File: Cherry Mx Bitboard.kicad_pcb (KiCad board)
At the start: 2 copper layers, 17.8 x 17.8 mm, 12 parts, among them P11 CONN_01X01, P12 CONN_01X01, P13 CONN_01X01, P14 CONN_01X01, P15 CONN_01X01, P16 CONN_01X01, P21 CONN_01X01, P22 CONN_01X01, P23 CONN_01X01, P24 CONN_01X01, SW1 SW_PUSH

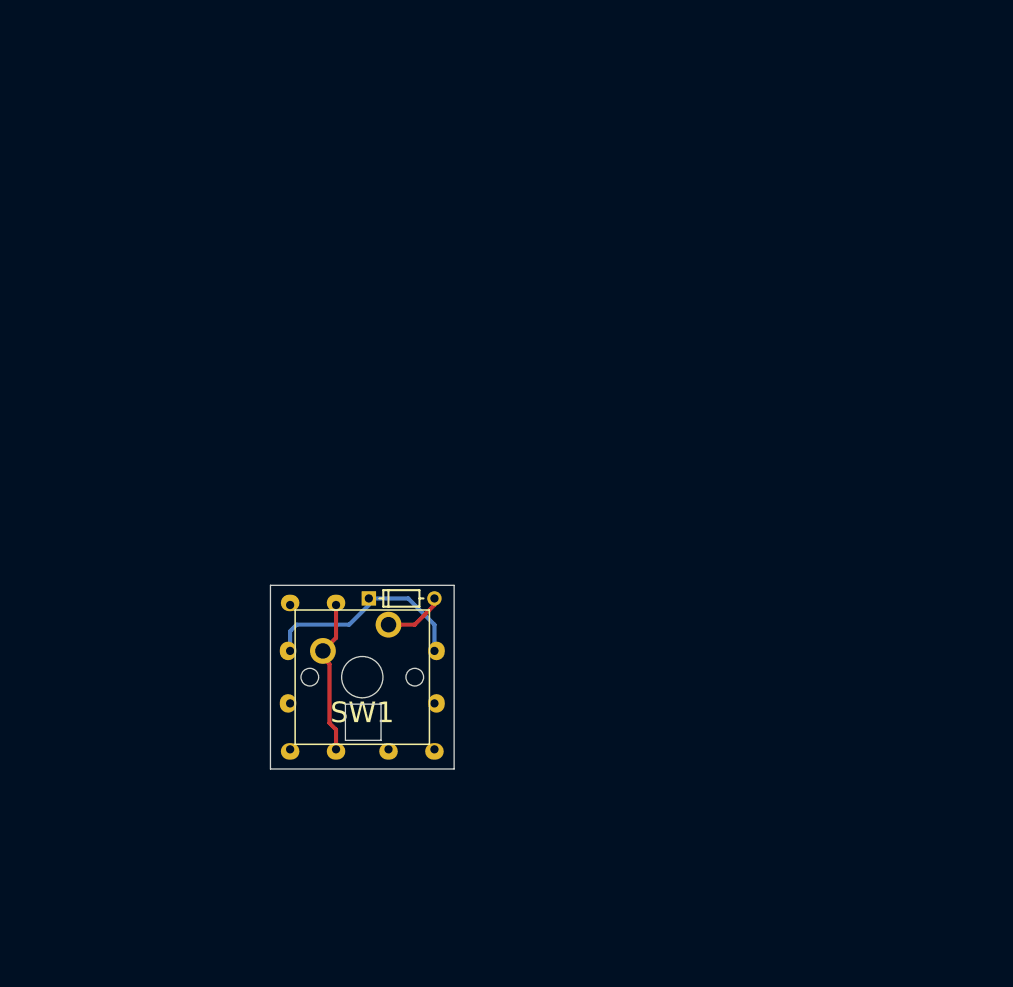
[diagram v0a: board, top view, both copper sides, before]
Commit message: first orderd
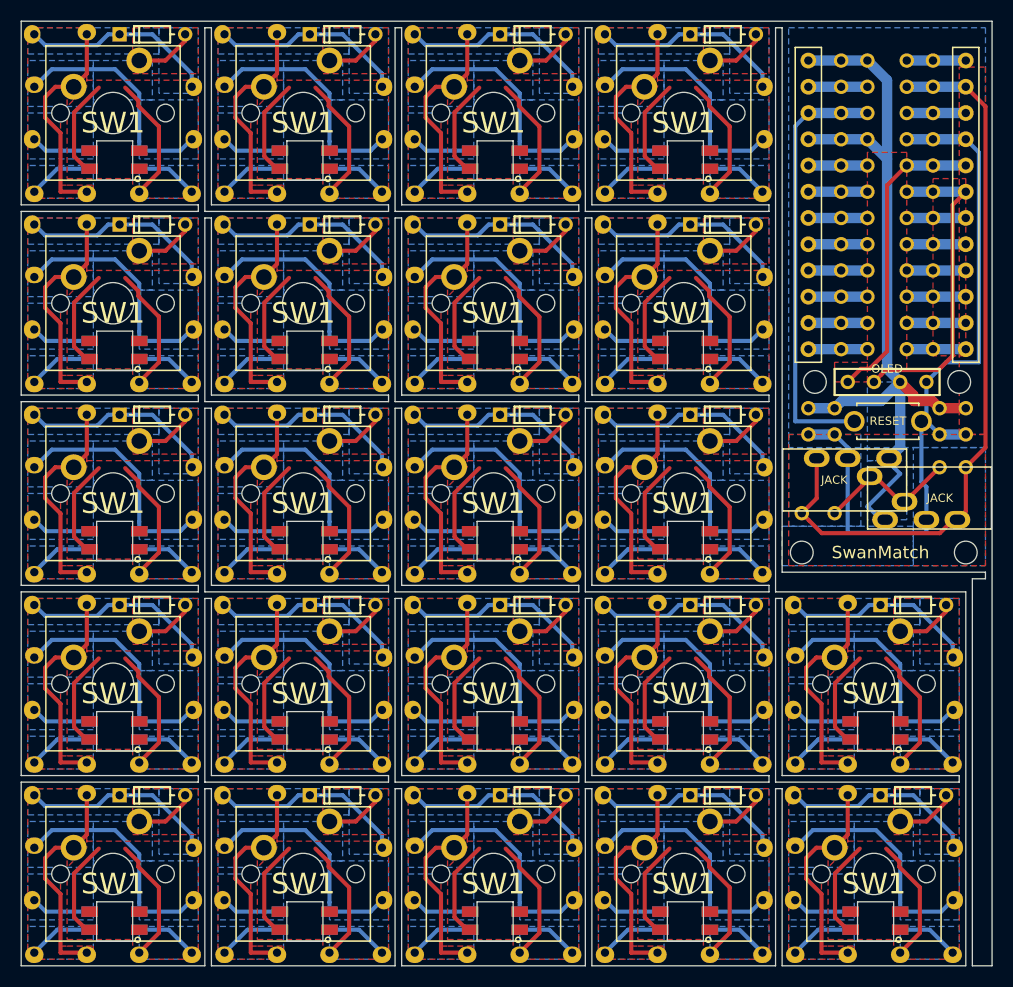
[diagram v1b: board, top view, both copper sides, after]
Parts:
- added A: CONN_01X01, MYLIB:1PIN_0.1, F.Cu at (170.8, 88.3)
- added A: CONN_01X01, MYLIB:1PIN_0.1, F.Cu at (160.7, 92.7)
- added D1: D, footprint:diode, B.Cu at (165.1, 120.0)
- added D1: D, footprint:diode, B.Cu at (91.4, 101.6)
- added D1: D, footprint:diode, B.Cu at (146.7, 83.2)
- added D1: D, footprint:diode, B.Cu at (128.3, 83.2)
- added D1: D, footprint:diode, B.Cu at (109.9, 83.2)
- added D1: D, footprint:diode, B.Cu at (91.4, 83.2)
- added D1: D, footprint:diode, B.Cu at (146.7, 64.8)
- added D1: D, footprint:diode, B.Cu at (128.3, 64.8)
- added D1: D, footprint:diode, B.Cu at (109.9, 64.8)
- added D1: D, footprint:diode, B.Cu at (91.4, 64.8)
- added D1: D, footprint:diode, B.Cu at (146.7, 46.4)
- added D1: D, footprint:diode, B.Cu at (165.1, 101.6)
- added D1: D, footprint:diode, B.Cu at (128.3, 46.4)
- added D1: D, footprint:diode, B.Cu at (109.9, 46.4)
- added D1: D, footprint:diode, B.Cu at (146.7, 120.0)
- added D1: D, footprint:diode, B.Cu at (128.3, 120.0)
- added D1: D, footprint:diode, B.Cu at (109.9, 120.0)
- added D1: D, footprint:diode, B.Cu at (91.4, 120.0)
- added D1: D, footprint:diode, B.Cu at (146.7, 101.6)
- added D1: D, footprint:diode, B.Cu at (128.3, 101.6)
- added D1: D, footprint:diode, B.Cu at (109.9, 101.6)
- added DATA: CONN_01X01, MYLIB:1PIN_0.1, F.Cu at (173.4, 88.3)
- added DATA: CONN_01X01, MYLIB:1PIN_0.1, F.Cu at (157.5, 92.7)
- added DT: CONN_01X01, MYLIB:1PIN_0.1, F.Cu at (167.6, 51.4)
- added HOLE_M2: VAL**, MYLIB:HOLE_M2, F.Cu at (172.7, 80.0)
- added HOLE_M2: VAL**, MYLIB:HOLE_M2, F.Cu at (158.8, 80.0)
- added HOLE_M2: VAL**, MYLIB:HOLE_M2, F.Cu at (173.4, 96.5)
- added HOLE_M2: VAL**, MYLIB:HOLE_M2, F.Cu at (157.5, 96.5)
- added JACK: MJ-4PP-9, MYLIB_REV:MJ-4PP-9_rev2, F.Cu at (155.6, 89.5)
- added JACK: MJ-4PP-9, MYLIB_REV:MJ-4PP-9_rev2, F.Cu at (175.8, 91.2)
- added OLED: OLED, MYLIB:MY_SIL-4, F.Cu at (161.9, 80.0)
- added P11: CONN_01X01, footprint:wirepad, F.Cu at (161.9, 120.0)
- added P11: CONN_01X01, footprint:wirepad, F.Cu at (88.3, 101.6)
- added P11: CONN_01X01, footprint:wirepad, F.Cu at (143.5, 83.2)
- added P11: CONN_01X01, footprint:wirepad, F.Cu at (125.1, 83.2)
- added P11: CONN_01X01, footprint:wirepad, F.Cu at (106.7, 83.2)
- added P11: CONN_01X01, footprint:wirepad, F.Cu at (88.3, 83.2)
- added P11: CONN_01X01, footprint:wirepad, F.Cu at (143.5, 64.8)
- added P11: CONN_01X01, footprint:wirepad, F.Cu at (125.1, 64.8)
- added P11: CONN_01X01, footprint:wirepad, F.Cu at (106.7, 64.8)
- added P11: CONN_01X01, footprint:wirepad, F.Cu at (88.3, 64.8)
- added P11: CONN_01X01, footprint:wirepad, F.Cu at (143.5, 46.4)
- added P11: CONN_01X01, footprint:wirepad, F.Cu at (161.9, 101.6)
- added P11: CONN_01X01, footprint:wirepad, F.Cu at (125.1, 46.4)
- added P11: CONN_01X01, footprint:wirepad, F.Cu at (106.7, 46.4)
- added P11: CONN_01X01, footprint:wirepad, F.Cu at (143.5, 120.0)
- added P11: CONN_01X01, footprint:wirepad, F.Cu at (125.1, 120.0)
- added P11: CONN_01X01, footprint:wirepad, F.Cu at (106.7, 120.0)
- added P11: CONN_01X01, footprint:wirepad, F.Cu at (88.3, 120.0)
- added P11: CONN_01X01, footprint:wirepad, F.Cu at (143.5, 101.6)
- added P11: CONN_01X01, footprint:wirepad, F.Cu at (125.1, 101.6)
- added P11: CONN_01X01, footprint:wirepad, F.Cu at (106.7, 101.6)
- added P12: CONN_01X01, footprint:wirepad, F.Cu at (156.8, 125.1)
- added P12: CONN_01X01, footprint:wirepad, F.Cu at (83.2, 106.7)
- added P12: CONN_01X01, footprint:wirepad, F.Cu at (138.4, 88.3)
- added P12: CONN_01X01, footprint:wirepad, F.Cu at (120.0, 88.3)
- added P12: CONN_01X01, footprint:wirepad, F.Cu at (101.6, 88.3)
- added P12: CONN_01X01, footprint:wirepad, F.Cu at (83.2, 88.3)
- added P12: CONN_01X01, footprint:wirepad, F.Cu at (138.4, 69.8)
- added P12: CONN_01X01, footprint:wirepad, F.Cu at (120.0, 69.8)
- added P12: CONN_01X01, footprint:wirepad, F.Cu at (101.6, 69.8)
- added P12: CONN_01X01, footprint:wirepad, F.Cu at (83.2, 69.8)
- added P12: CONN_01X01, footprint:wirepad, F.Cu at (138.4, 51.4)
- added P12: CONN_01X01, footprint:wirepad, F.Cu at (156.8, 106.7)
- added P12: CONN_01X01, footprint:wirepad, F.Cu at (120.0, 51.4)
- added P12: CONN_01X01, footprint:wirepad, F.Cu at (101.6, 51.4)
- added P12: CONN_01X01, footprint:wirepad, F.Cu at (138.4, 125.1)
- added P12: CONN_01X01, footprint:wirepad, F.Cu at (120.0, 125.1)
- added P12: CONN_01X01, footprint:wirepad, F.Cu at (101.6, 125.1)
- added P12: CONN_01X01, footprint:wirepad, F.Cu at (83.2, 125.1)
- added P12: CONN_01X01, footprint:wirepad, F.Cu at (138.4, 106.7)
- added P12: CONN_01X01, footprint:wirepad, F.Cu at (120.0, 106.7)
- added P12: CONN_01X01, footprint:wirepad, F.Cu at (101.6, 106.7)
- added P13: CONN_01X01, footprint:wirepad, F.Cu at (161.9, 116.8)
- added P13: CONN_01X01, footprint:wirepad, F.Cu at (88.3, 116.8)
- added P13: CONN_01X01, footprint:wirepad, F.Cu at (143.5, 98.4)
- added P13: CONN_01X01, footprint:wirepad, F.Cu at (125.1, 98.4)
- added P13: CONN_01X01, footprint:wirepad, F.Cu at (106.7, 98.4)
- added P13: CONN_01X01, footprint:wirepad, F.Cu at (88.3, 98.4)
- added P13: CONN_01X01, footprint:wirepad, F.Cu at (143.5, 80.0)
- added P13: CONN_01X01, footprint:wirepad, F.Cu at (125.1, 80.0)
- added P13: CONN_01X01, footprint:wirepad, F.Cu at (106.7, 80.0)
- added P13: CONN_01X01, footprint:wirepad, F.Cu at (88.3, 80.0)
- added P13: CONN_01X01, footprint:wirepad, F.Cu at (143.5, 61.6)
- added P13: CONN_01X01, footprint:wirepad, F.Cu at (161.9, 135.3)
- added P13: CONN_01X01, footprint:wirepad, F.Cu at (125.1, 61.6)
- added P13: CONN_01X01, footprint:wirepad, F.Cu at (106.7, 61.6)
- added P13: CONN_01X01, footprint:wirepad, F.Cu at (143.5, 135.3)
- added P13: CONN_01X01, footprint:wirepad, F.Cu at (125.1, 135.3)
- added P13: CONN_01X01, footprint:wirepad, F.Cu at (106.7, 135.3)
- added P13: CONN_01X01, footprint:wirepad, F.Cu at (88.3, 135.3)
- added P13: CONN_01X01, footprint:wirepad, F.Cu at (143.5, 116.8)
- added P13: CONN_01X01, footprint:wirepad, F.Cu at (125.1, 116.8)
- added P13: CONN_01X01, footprint:wirepad, F.Cu at (106.7, 116.8)
- added P14: CONN_01X01, footprint:wirepad, F.Cu at (156.8, 116.8)
- added P14: CONN_01X01, footprint:wirepad, F.Cu at (83.2, 116.8)
- added P14: CONN_01X01, footprint:wirepad, F.Cu at (138.4, 98.4)
- added P14: CONN_01X01, footprint:wirepad, F.Cu at (120.0, 98.4)
- added P14: CONN_01X01, footprint:wirepad, F.Cu at (101.6, 98.4)
- added P14: CONN_01X01, footprint:wirepad, F.Cu at (83.2, 98.4)
- added P14: CONN_01X01, footprint:wirepad, F.Cu at (138.4, 80.0)
- added P14: CONN_01X01, footprint:wirepad, F.Cu at (120.0, 80.0)
- added P14: CONN_01X01, footprint:wirepad, F.Cu at (101.6, 80.0)
- added P14: CONN_01X01, footprint:wirepad, F.Cu at (83.2, 80.0)
- added P14: CONN_01X01, footprint:wirepad, F.Cu at (138.4, 61.6)
- added P14: CONN_01X01, footprint:wirepad, F.Cu at (156.8, 135.3)
- added P14: CONN_01X01, footprint:wirepad, F.Cu at (120.0, 61.6)
- added P14: CONN_01X01, footprint:wirepad, F.Cu at (101.6, 61.6)
- added P14: CONN_01X01, footprint:wirepad, F.Cu at (138.4, 135.3)
- added P14: CONN_01X01, footprint:wirepad, F.Cu at (120.0, 135.3)
- added P14: CONN_01X01, footprint:wirepad, F.Cu at (101.6, 135.3)
- added P14: CONN_01X01, footprint:wirepad, F.Cu at (83.2, 135.3)
- added P14: CONN_01X01, footprint:wirepad, F.Cu at (138.4, 116.8)
- added P14: CONN_01X01, footprint:wirepad, F.Cu at (120.0, 116.8)
- added P14: CONN_01X01, footprint:wirepad, F.Cu at (101.6, 116.8)
- added P15: CONN_01X01, footprint:wirepad, F.Cu at (172.1, 116.8)
- added P15: CONN_01X01, footprint:wirepad, F.Cu at (98.4, 116.8)
- added P15: CONN_01X01, footprint:wirepad, F.Cu at (153.7, 98.4)
- added P15: CONN_01X01, footprint:wirepad, F.Cu at (135.3, 98.4)
- added P15: CONN_01X01, footprint:wirepad, F.Cu at (116.8, 98.4)
- added P15: CONN_01X01, footprint:wirepad, F.Cu at (98.4, 98.4)
- added P15: CONN_01X01, footprint:wirepad, F.Cu at (153.7, 80.0)
- added P15: CONN_01X01, footprint:wirepad, F.Cu at (135.3, 80.0)
- added P15: CONN_01X01, footprint:wirepad, F.Cu at (116.8, 80.0)
- added P15: CONN_01X01, footprint:wirepad, F.Cu at (98.4, 80.0)
- added P15: CONN_01X01, footprint:wirepad, F.Cu at (153.7, 61.6)
- added P15: CONN_01X01, footprint:wirepad, F.Cu at (172.1, 135.3)
- added P15: CONN_01X01, footprint:wirepad, F.Cu at (135.3, 61.6)
- added P15: CONN_01X01, footprint:wirepad, F.Cu at (116.8, 61.6)
- added P15: CONN_01X01, footprint:wirepad, F.Cu at (153.7, 135.3)
- added P15: CONN_01X01, footprint:wirepad, F.Cu at (135.3, 135.3)
- added P15: CONN_01X01, footprint:wirepad, F.Cu at (116.8, 135.3)
- added P15: CONN_01X01, footprint:wirepad, F.Cu at (98.4, 135.3)
- added P15: CONN_01X01, footprint:wirepad, F.Cu at (153.7, 116.8)
- added P15: CONN_01X01, footprint:wirepad, F.Cu at (135.3, 116.8)
- added P15: CONN_01X01, footprint:wirepad, F.Cu at (116.8, 116.8)
- added P16: CONN_01X01, footprint:wirepad, F.Cu at (167.0, 116.8)
- added P16: CONN_01X01, footprint:wirepad, F.Cu at (93.3, 116.8)
- added P16: CONN_01X01, footprint:wirepad, F.Cu at (148.6, 98.4)
- added P16: CONN_01X01, footprint:wirepad, F.Cu at (130.2, 98.4)
- added P16: CONN_01X01, footprint:wirepad, F.Cu at (111.8, 98.4)
- added P16: CONN_01X01, footprint:wirepad, F.Cu at (93.3, 98.4)
- added P16: CONN_01X01, footprint:wirepad, F.Cu at (148.6, 80.0)
- added P16: CONN_01X01, footprint:wirepad, F.Cu at (130.2, 80.0)
- added P16: CONN_01X01, footprint:wirepad, F.Cu at (111.8, 80.0)
- added P16: CONN_01X01, footprint:wirepad, F.Cu at (93.3, 80.0)
- added P16: CONN_01X01, footprint:wirepad, F.Cu at (148.6, 61.6)
- added P16: CONN_01X01, footprint:wirepad, F.Cu at (167.0, 135.3)
- added P16: CONN_01X01, footprint:wirepad, F.Cu at (130.2, 61.6)
- added P16: CONN_01X01, footprint:wirepad, F.Cu at (111.8, 61.6)
- added P16: CONN_01X01, footprint:wirepad, F.Cu at (148.6, 135.3)
- added P16: CONN_01X01, footprint:wirepad, F.Cu at (130.2, 135.3)
- added P16: CONN_01X01, footprint:wirepad, F.Cu at (111.8, 135.3)
- added P16: CONN_01X01, footprint:wirepad, F.Cu at (93.3, 135.3)
- added P16: CONN_01X01, footprint:wirepad, F.Cu at (148.6, 116.8)
- added P16: CONN_01X01, footprint:wirepad, F.Cu at (130.2, 116.8)
- added P16: CONN_01X01, footprint:wirepad, F.Cu at (111.8, 116.8)
- added P2: CONN_01X01, MYLIB:1PIN_0.1, F.Cu at (173.4, 85.1)
- added P2: CONN_01X01, MYLIB:1PIN_0.1, F.Cu at (167.6, 64.1)
- added P2: CONN_01X01, MYLIB:1PIN_0.1, F.Cu at (167.6, 66.7)
- added P2: CONN_01X01, MYLIB:1PIN_0.1, F.Cu at (170.2, 69.2)
- added P2: CONN_01X01, MYLIB:1PIN_0.1, F.Cu at (167.6, 69.2)
- added P2: CONN_01X01, MYLIB:1PIN_0.1, F.Cu at (170.2, 64.1)
- added P2: CONN_01X01, MYLIB:1PIN_0.1, F.Cu at (170.2, 71.8)
- added P2: CONN_01X01, MYLIB:1PIN_0.1, F.Cu at (167.6, 71.8)
- added P2: CONN_01X01, MYLIB:1PIN_0.1, F.Cu at (170.2, 74.3)
- added P2: CONN_01X01, MYLIB:1PIN_0.1, F.Cu at (167.6, 74.3)
- added P2: CONN_01X01, MYLIB:1PIN_0.1, F.Cu at (170.2, 76.8)
- added P2: CONN_01X01, MYLIB:1PIN_0.1, F.Cu at (170.8, 85.1)
- added P2: CONN_01X01, MYLIB:1PIN_0.1, F.Cu at (167.6, 76.8)
- added P2: CONN_01X01, MYLIB:1PIN_0.1, F.Cu at (161.3, 74.3)
- added P2: CONN_01X01, MYLIB:1PIN_0.1, F.Cu at (163.8, 76.8)
- added P2: CONN_01X01, MYLIB:1PIN_0.1, F.Cu at (163.8, 74.3)
- added P2: CONN_01X01, MYLIB:1PIN_0.1, F.Cu at (163.8, 71.8)
- added P2: CONN_01X01, MYLIB:1PIN_0.1, F.Cu at (161.3, 71.8)
- added P2: CONN_01X01, MYLIB:1PIN_0.1, F.Cu at (161.3, 76.8)
- added P2: CONN_01X01, MYLIB:1PIN_0.1, F.Cu at (161.3, 69.2)
- added P2: CONN_01X01, MYLIB:1PIN_0.1, F.Cu at (163.8, 69.2)
- added P2: CONN_01X01, MYLIB:1PIN_0.1, F.Cu at (161.3, 66.7)
- added P2: CONN_01X01, MYLIB:1PIN_0.1, F.Cu at (170.8, 82.5)
- added P2: CONN_01X01, MYLIB:1PIN_0.1, F.Cu at (163.8, 66.7)
- added P2: CONN_01X01, MYLIB:1PIN_0.1, F.Cu at (161.3, 64.1)
- added P2: CONN_01X01, MYLIB:1PIN_0.1, F.Cu at (163.8, 64.1)
- added P2: CONN_01X01, MYLIB:1PIN_0.1, F.Cu at (161.3, 61.6)
- added P2: CONN_01X01, MYLIB:1PIN_0.1, F.Cu at (167.6, 59.1)
- added P2: CONN_01X01, MYLIB:1PIN_0.1, F.Cu at (167.6, 61.6)
- added P2: CONN_01X01, MYLIB:1PIN_0.1, F.Cu at (167.6, 48.9)
- added P2: CONN_01X01, MYLIB:1PIN_0.1, F.Cu at (167.6, 54.0)
- added P2: CONN_01X01, MYLIB:1PIN_0.1, F.Cu at (167.6, 56.5)
- added P2: CONN_01X01, MYLIB:1PIN_0.1, F.Cu at (163.8, 59.1)
- added P2: CONN_01X01, MYLIB:1PIN_0.1, F.Cu at (173.4, 82.5)
- added P2: CONN_01X01, MYLIB:1PIN_0.1, F.Cu at (163.8, 61.6)
- added P2: CONN_01X01, MYLIB:1PIN_0.1, F.Cu at (163.8, 48.9)
- added P2: CONN_01X01, MYLIB:1PIN_0.1, F.Cu at (163.8, 54.0)
- added P2: CONN_01X01, MYLIB:1PIN_0.1, F.Cu at (163.8, 56.5)
- added P2: CONN_01X01, MYLIB:1PIN_0.1, F.Cu at (163.8, 51.4)
- added P2: CONN_01X01, MYLIB:1PIN_0.1, F.Cu at (170.2, 61.6)
- added P2: CONN_01X01, MYLIB:1PIN_0.1, F.Cu at (170.2, 48.9)
- added P2: CONN_01X01, MYLIB:1PIN_0.1, F.Cu at (170.2, 59.1)
- added P2: CONN_01X01, MYLIB:1PIN_0.1, F.Cu at (170.2, 54.0)
- added P2: CONN_01X01, MYLIB:1PIN_0.1, F.Cu at (170.2, 51.4)
- added P2: CONN_01X01, MYLIB:1PIN_0.1, F.Cu at (158.1, 85.1)
- added P2: CONN_01X01, MYLIB:1PIN_0.1, F.Cu at (170.2, 56.5)
- added P2: CONN_01X01, MYLIB:1PIN_0.1, F.Cu at (161.3, 59.1)
- added P2: CONN_01X01, MYLIB:1PIN_0.1, F.Cu at (161.3, 56.5)
- added P2: CONN_01X01, MYLIB:1PIN_0.1, F.Cu at (161.3, 54.0)
- added P2: CONN_01X01, MYLIB:1PIN_0.1, F.Cu at (161.3, 51.4)
- added P2: CONN_01X01, MYLIB:1PIN_0.1, F.Cu at (161.3, 48.9)
- added P2: CONN_01X01, MYLIB:1PIN_0.1, F.Cu at (160.7, 85.1)
- added P2: CONN_01X01, MYLIB:1PIN_0.1, F.Cu at (158.1, 82.5)
- added P2: CONN_01X01, MYLIB:1PIN_0.1, F.Cu at (160.7, 82.5)
- added P2: CONN_01X01, MYLIB:1PIN_0.1, F.Cu at (170.2, 66.7)
- added P21: CONN_01X01, footprint:wirepad, F.Cu at (172.1, 111.8)
- added P21: CONN_01X01, footprint:wirepad, F.Cu at (98.4, 111.8)
- added P21: CONN_01X01, footprint:wirepad, F.Cu at (153.7, 93.3)
- added P21: CONN_01X01, footprint:wirepad, F.Cu at (135.3, 93.3)
- added P21: CONN_01X01, footprint:wirepad, F.Cu at (116.8, 93.3)
- added P21: CONN_01X01, footprint:wirepad, F.Cu at (98.4, 93.3)
- added P21: CONN_01X01, footprint:wirepad, F.Cu at (153.7, 74.9)
- added P21: CONN_01X01, footprint:wirepad, F.Cu at (135.3, 74.9)
- added P21: CONN_01X01, footprint:wirepad, F.Cu at (116.8, 74.9)
- added P21: CONN_01X01, footprint:wirepad, F.Cu at (98.4, 74.9)
- added P21: CONN_01X01, footprint:wirepad, F.Cu at (153.7, 56.5)
- added P21: CONN_01X01, footprint:wirepad, F.Cu at (172.1, 130.2)
- added P21: CONN_01X01, footprint:wirepad, F.Cu at (135.3, 56.5)
- added P21: CONN_01X01, footprint:wirepad, F.Cu at (116.8, 56.5)
- added P21: CONN_01X01, footprint:wirepad, F.Cu at (153.7, 130.2)
- added P21: CONN_01X01, footprint:wirepad, F.Cu at (135.3, 130.2)
- added P21: CONN_01X01, footprint:wirepad, F.Cu at (116.8, 130.2)
- added P21: CONN_01X01, footprint:wirepad, F.Cu at (98.4, 130.2)
- added P21: CONN_01X01, footprint:wirepad, F.Cu at (153.7, 111.8)
- added P21: CONN_01X01, footprint:wirepad, F.Cu at (135.3, 111.8)
- added P21: CONN_01X01, footprint:wirepad, F.Cu at (116.8, 111.8)
- added P22: CONN_01X01, footprint:wirepad, F.Cu at (172.1, 106.7)
- added P22: CONN_01X01, footprint:wirepad, F.Cu at (98.4, 106.7)
- added P22: CONN_01X01, footprint:wirepad, F.Cu at (153.7, 88.3)
- added P22: CONN_01X01, footprint:wirepad, F.Cu at (135.3, 88.3)
- added P22: CONN_01X01, footprint:wirepad, F.Cu at (116.8, 88.3)
- added P22: CONN_01X01, footprint:wirepad, F.Cu at (98.4, 88.3)
- added P22: CONN_01X01, footprint:wirepad, F.Cu at (153.7, 69.8)
- added P22: CONN_01X01, footprint:wirepad, F.Cu at (135.3, 69.8)
- added P22: CONN_01X01, footprint:wirepad, F.Cu at (116.8, 69.8)
- added P22: CONN_01X01, footprint:wirepad, F.Cu at (98.4, 69.8)
- added P22: CONN_01X01, footprint:wirepad, F.Cu at (153.7, 51.4)
- added P22: CONN_01X01, footprint:wirepad, F.Cu at (172.1, 125.1)
- added P22: CONN_01X01, footprint:wirepad, F.Cu at (135.3, 51.4)
- added P22: CONN_01X01, footprint:wirepad, F.Cu at (116.8, 51.4)
- added P22: CONN_01X01, footprint:wirepad, F.Cu at (153.7, 125.1)
- added P22: CONN_01X01, footprint:wirepad, F.Cu at (135.3, 125.1)
- added P22: CONN_01X01, footprint:wirepad, F.Cu at (116.8, 125.1)
- added P22: CONN_01X01, footprint:wirepad, F.Cu at (98.4, 125.1)
- added P22: CONN_01X01, footprint:wirepad, F.Cu at (153.7, 106.7)
- added P22: CONN_01X01, footprint:wirepad, F.Cu at (135.3, 106.7)
- added P22: CONN_01X01, footprint:wirepad, F.Cu at (116.8, 106.7)
- added P23: CONN_01X01, footprint:wirepad, F.Cu at (156.8, 120.0)
- added P23: CONN_01X01, footprint:wirepad, F.Cu at (83.2, 101.6)
- added P23: CONN_01X01, footprint:wirepad, F.Cu at (138.4, 83.2)
- added P23: CONN_01X01, footprint:wirepad, F.Cu at (120.0, 83.2)
- added P23: CONN_01X01, footprint:wirepad, F.Cu at (101.6, 83.2)
- added P23: CONN_01X01, footprint:wirepad, F.Cu at (83.2, 83.2)
- added P23: CONN_01X01, footprint:wirepad, F.Cu at (138.4, 64.8)
- added P23: CONN_01X01, footprint:wirepad, F.Cu at (120.0, 64.8)
- added P23: CONN_01X01, footprint:wirepad, F.Cu at (101.6, 64.8)
- added P23: CONN_01X01, footprint:wirepad, F.Cu at (83.2, 64.8)
- added P23: CONN_01X01, footprint:wirepad, F.Cu at (138.4, 46.4)
- added P23: CONN_01X01, footprint:wirepad, F.Cu at (156.8, 101.6)
- added P23: CONN_01X01, footprint:wirepad, F.Cu at (120.0, 46.4)
- added P23: CONN_01X01, footprint:wirepad, F.Cu at (101.6, 46.4)
- added P23: CONN_01X01, footprint:wirepad, F.Cu at (138.4, 120.0)
- added P23: CONN_01X01, footprint:wirepad, F.Cu at (120.0, 120.0)
- added P23: CONN_01X01, footprint:wirepad, F.Cu at (101.6, 120.0)
- added P23: CONN_01X01, footprint:wirepad, F.Cu at (83.2, 120.0)
- added P23: CONN_01X01, footprint:wirepad, F.Cu at (138.4, 101.6)
- added P23: CONN_01X01, footprint:wirepad, F.Cu at (120.0, 101.6)
- added P23: CONN_01X01, footprint:wirepad, F.Cu at (101.6, 101.6)
- added P24: CONN_01X01, footprint:wirepad, F.Cu at (156.8, 130.2)
- added P24: CONN_01X01, footprint:wirepad, F.Cu at (83.2, 111.8)
- added P24: CONN_01X01, footprint:wirepad, F.Cu at (138.4, 93.3)
- added P24: CONN_01X01, footprint:wirepad, F.Cu at (120.0, 93.3)
- added P24: CONN_01X01, footprint:wirepad, F.Cu at (101.6, 93.3)
- added P24: CONN_01X01, footprint:wirepad, F.Cu at (83.2, 93.3)
- added P24: CONN_01X01, footprint:wirepad, F.Cu at (138.4, 74.9)
- added P24: CONN_01X01, footprint:wirepad, F.Cu at (120.0, 74.9)
- added P24: CONN_01X01, footprint:wirepad, F.Cu at (101.6, 74.9)
- added P24: CONN_01X01, footprint:wirepad, F.Cu at (83.2, 74.9)
- added P24: CONN_01X01, footprint:wirepad, F.Cu at (138.4, 56.5)
- added P24: CONN_01X01, footprint:wirepad, F.Cu at (156.8, 111.8)
- added P24: CONN_01X01, footprint:wirepad, F.Cu at (120.0, 56.5)
- added P24: CONN_01X01, footprint:wirepad, F.Cu at (101.6, 56.5)
- added P24: CONN_01X01, footprint:wirepad, F.Cu at (138.4, 130.2)
- added P24: CONN_01X01, footprint:wirepad, F.Cu at (120.0, 130.2)
- added P24: CONN_01X01, footprint:wirepad, F.Cu at (101.6, 130.2)
- added P24: CONN_01X01, footprint:wirepad, F.Cu at (83.2, 130.2)
- added P24: CONN_01X01, footprint:wirepad, F.Cu at (138.4, 111.8)
- added P24: CONN_01X01, footprint:wirepad, F.Cu at (120.0, 111.8)
- added P24: CONN_01X01, footprint:wirepad, F.Cu at (101.6, 111.8)
- added RESET1: RESET, MYLIB:SW_3.5x6.0_TH, F.Cu at (165.8, 83.8)
- added SW1: SW_PUSH, footprint:switch, F.Cu at (164.5, 109.2)
- added SW1: SW_PUSH, footprint:switch, F.Cu at (90.8, 109.2)
- added SW1: SW_PUSH, footprint:switch, F.Cu at (146.1, 90.8)
- added SW1: SW_PUSH, footprint:switch, F.Cu at (127.6, 90.8)
- added SW1: SW_PUSH, footprint:switch, F.Cu at (109.2, 90.8)
- added SW1: SW_PUSH, footprint:switch, F.Cu at (90.8, 90.8)
- added SW1: SW_PUSH, footprint:switch, F.Cu at (146.1, 72.4)
- added SW1: SW_PUSH, footprint:switch, F.Cu at (127.6, 72.4)
- added SW1: SW_PUSH, footprint:switch, F.Cu at (109.2, 72.4)
- added SW1: SW_PUSH, footprint:switch, F.Cu at (90.8, 72.4)
- added SW1: SW_PUSH, footprint:switch, F.Cu at (146.1, 54.0)
- added SW1: SW_PUSH, footprint:switch, F.Cu at (164.5, 127.6)
- added SW1: SW_PUSH, footprint:switch, F.Cu at (127.6, 54.0)
- added SW1: SW_PUSH, footprint:switch, F.Cu at (109.2, 54.0)
- added SW1: SW_PUSH, footprint:switch, F.Cu at (146.1, 127.6)
- added SW1: SW_PUSH, footprint:switch, F.Cu at (127.6, 127.6)
- added SW1: SW_PUSH, footprint:switch, F.Cu at (109.2, 127.6)
- added SW1: SW_PUSH, footprint:switch, F.Cu at (90.8, 127.6)
- added SW1: SW_PUSH, footprint:switch, F.Cu at (146.1, 109.2)
- added SW1: SW_PUSH, footprint:switch, F.Cu at (127.6, 109.2)
- added SW1: SW_PUSH, footprint:switch, F.Cu at (109.2, 109.2)
- added U1: SK6812mini, sk6812:SK6812MINI_rev, F.Cu at (164.6, 113.7)
- added U1: SK6812mini, sk6812:SK6812MINI_rev, F.Cu at (90.9, 113.7)
- added U1: SK6812mini, sk6812:SK6812MINI_rev, F.Cu at (146.2, 95.3)
- added U1: SK6812mini, sk6812:SK6812MINI_rev, F.Cu at (127.8, 95.3)
- added U1: SK6812mini, sk6812:SK6812MINI_rev, F.Cu at (109.4, 95.3)
- added U1: SK6812mini, sk6812:SK6812MINI_rev, F.Cu at (90.9, 95.3)
- added U1: SK6812mini, sk6812:SK6812MINI_rev, F.Cu at (146.2, 76.9)
- added U1: SK6812mini, sk6812:SK6812MINI_rev, F.Cu at (127.8, 76.9)
- added U1: SK6812mini, sk6812:SK6812MINI_rev, F.Cu at (109.4, 76.9)
- added U1: SK6812mini, sk6812:SK6812MINI_rev, F.Cu at (90.9, 76.9)
- added U1: SK6812mini, sk6812:SK6812MINI_rev, F.Cu at (146.2, 58.5)
- added U1: SK6812mini, sk6812:SK6812MINI_rev, F.Cu at (164.6, 132.2)
- added U1: SK6812mini, sk6812:SK6812MINI_rev, F.Cu at (127.8, 58.5)
- added U1: SK6812mini, sk6812:SK6812MINI_rev, F.Cu at (109.4, 58.5)
- added U1: SK6812mini, sk6812:SK6812MINI_rev, F.Cu at (90.9, 58.5)
- added U1: SK6812mini, sk6812:SK6812MINI_rev, F.Cu at (146.2, 132.2)
- added U1: SK6812mini, sk6812:SK6812MINI_rev, F.Cu at (127.8, 132.2)
- added U1: SK6812mini, sk6812:SK6812MINI_rev, F.Cu at (109.4, 132.2)
- added U1: SK6812mini, sk6812:SK6812MINI_rev, F.Cu at (90.9, 132.2)
- added U1: SK6812mini, sk6812:SK6812MINI_rev, F.Cu at (146.2, 113.7)
- added U1: SK6812mini, sk6812:SK6812MINI_rev, F.Cu at (127.8, 113.7)
- added U1: SK6812mini, sk6812:SK6812MINI_rev, F.Cu at (109.4, 113.7)
- added U2: ProMicro, MYLIB:ProMicro_rev, B.Cu at (165.7, 62.9)
- moved P23 64.6 mm to (83.2, 46.4)
- moved P11 60.3 mm to (88.3, 46.4)
- moved P24 60.0 mm to (83.2, 56.5)
- moved D1 59.7 mm to (91.4, 46.4)
- moved SW1 59.7 mm to (90.8, 54.0)
- moved P21 59.4 mm to (98.4, 56.5)
- moved P22 59.4 mm to (98.4, 51.4)
- moved P14 59.4 mm to (83.2, 61.6)
- moved P13 59.1 mm to (88.3, 61.6)
- moved P16 59.1 mm to (93.3, 61.6)
- moved P15 58.9 mm to (98.4, 61.6)
- moved P12 55.9 mm to (83.2, 51.4)
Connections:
- P12 pad 1: /1 -> Net-(U1-Pad3)
- P14 pad 1: /1 -> Net-(U1-Pad2)
- P15 pad 1: /1 -> Net-(U1-Pad4)
- P16 pad 1: /1 -> Net-(U1-Pad2)
- P21 pad 1: /2 -> Net-(U1-Pad3)
- P24 pad 1: /2 -> Net-(U1-Pad1)
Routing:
- net Net-(U1-Pad2): track 0.00 -> 619.1 mm
- net Net-(U1-Pad3): track 0.00 -> 504.4 mm
- net /1: track 15.0 -> 478.1 mm
- net /2: track 21.2 -> 417.1 mm
- net Net-(U1-Pad4): track 0.00 -> 132.0 mm
- net Net-(U1-Pad1): track 0.00 -> 128.0 mm
- net Net-(D1-Pad2): track 5.87 -> 129.1 mm
- net GND: track 0.00 -> 85.2 mm
- net VCC: track 0.00 -> 81.4 mm
- net DATA: track 0.00 -> 71.9 mm
- net (no net): track 0.00 -> 47.9 mm
- net RESET: track 0.00 -> 41.7 mm
- net SCL: track 0.00 -> 30.8 mm
- net SDA: track 0.00 -> 29.5 mm
- net Net-(PM21-Pad1): track 0.00 -> 5.72 mm
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- added copper zone on F.Cu, net /1
- added copper zone on B.Cu, net /2
- added copper zone on F.Cu, net DATA
- added copper zone on B.Cu, net GND
- added copper zone on F.Cu, net Net-(D1-Pad2)
- added copper zone on B.Cu, net Net-(U1-Pad1)
- added copper zone on B.Cu, net Net-(U1-Pad2)
- added copper zone on F.Cu, net Net-(U1-Pad2)
- added copper zone on B.Cu, net Net-(U1-Pad3)
- added copper zone on B.Cu, net Net-(U1-Pad4)
- added copper zone on F.Cu, net SCL
- added copper zone on F.Cu, net SDA
- added copper zone on B.Cu, net VCC
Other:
- board size 17.8 x 17.8 mm -> 94 x 91.4 mm
- board text added: "+"
- board text added: "-"
- board text added: "10"
- board text added: "14"
- board text added: "15"
- board text added: "16"
- board text added: "4"
- board text added: "5"
- board text added: "6"
- board text added: "7"
- board text added: "8"
- board text added: "9"
- board text added: "A0"
- board text added: "A1"
- board text added: "A2"
- board text added: "A3"
- board text added: "C"
- board text added: "DI"
- board text added: "DO"
- board text added: "DT"
- board text added: "LED"
- board text added: "R"
- board text added: "RST"
- board text added: "SCL"
- board text added: "SDA"
- board text added: "SHIROTRON"
- board text added: "SwanMatch"
- board text removed: "1"
- board text removed: "2"
